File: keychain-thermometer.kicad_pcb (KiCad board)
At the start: 2 copper layers, 23.5 x 27.4 mm, 16 parts, among them J1 Conn_01x06_Pin, SW1 SW_Push_Dual, U1 ATtiny85V-10S

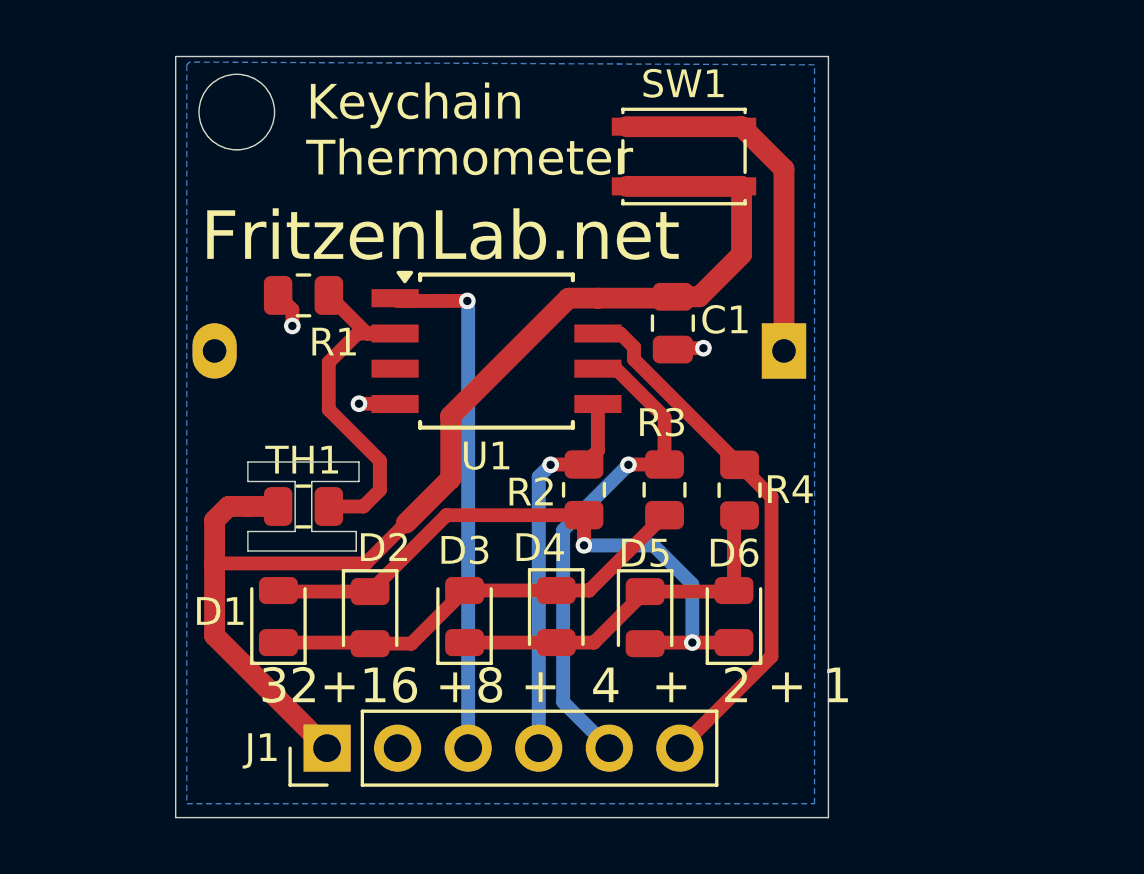
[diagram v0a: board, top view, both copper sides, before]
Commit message: Edited - r01 created
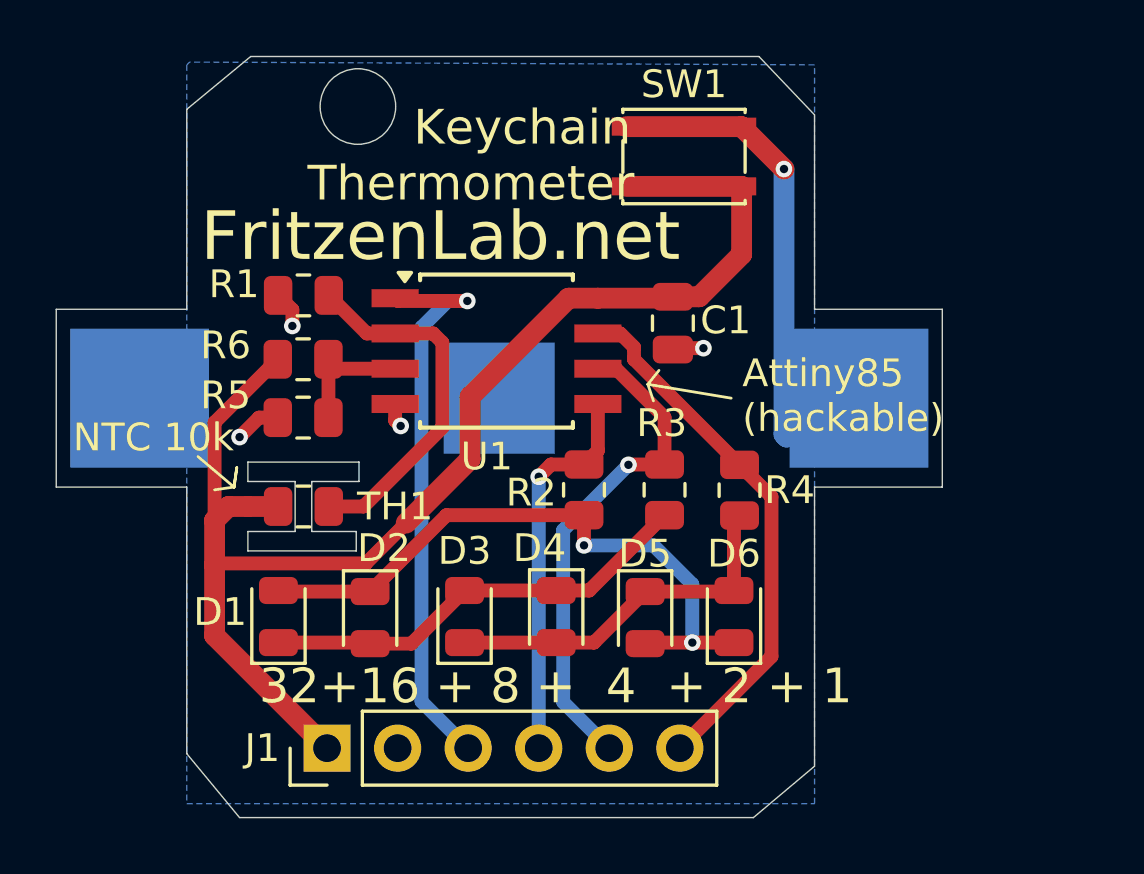
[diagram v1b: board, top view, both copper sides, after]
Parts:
- added R5: 10k, Resistor_SMD:R_0805_2012Metric, F.Cu at (68.0, 57.2)
- added R6: 10k, Resistor_SMD:R_0805_2012Metric, F.Cu at (68.0, 55.1)
- BT1: footprint Battery:Battery_Panasonic_CR2032-HFN_Horizontal_CircularHoles -> Battery:BatteryHolder_Multicomp_BC-2001_1x2032
- moved BT1 10.4 mm to (75.0, 56.5)
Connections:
- U1 pad 3: unconnected-(U1-XTAL2/PB4-Pad3) -> REF
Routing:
- net VCC: track 43.9 -> 50.6 mm
- net Net-(BT1-+): track 12.9 -> 19.2 mm, vias 0 -> 1
- net REF: track 0.00 -> 4.64 mm
- net PB5-reset: track 18.8 -> 20.6 mm
- net GND: track 3.74 -> 4.97 mm, vias 3 -> 4
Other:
- board size 23.5 x 27.4 mm -> 31.9 x 27.4 mm
- board text added: "32+16 + 8 + 4 + 2 + 1"
- board text added: "Attiny85 (hackable)"
- board text added: "NTC 10k"
- board text removed: "32+16 +8 + 4 + 2 + 1"
